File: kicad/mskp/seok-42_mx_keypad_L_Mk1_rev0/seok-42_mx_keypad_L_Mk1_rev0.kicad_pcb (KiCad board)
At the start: 2 copper layers, 162 x 117 mm, 44 parts, among them J1 Conn_01x12_Socket, SW1 Switch, SW10 Switch, SW11 Switch, SW12 Switch, SW13 Switch, SW14 Switch, SW15 Switch, SW16 Switch, SW17 Switch, SW18 Switch, SW19 Switch, SW2 Switch, SW20 Switch, SW21 Switch, SW3 Switch, SW4 Switch, SW5 Switch, SW6 Switch, SW7 Switch, SW8 Switch, SW9 Switch

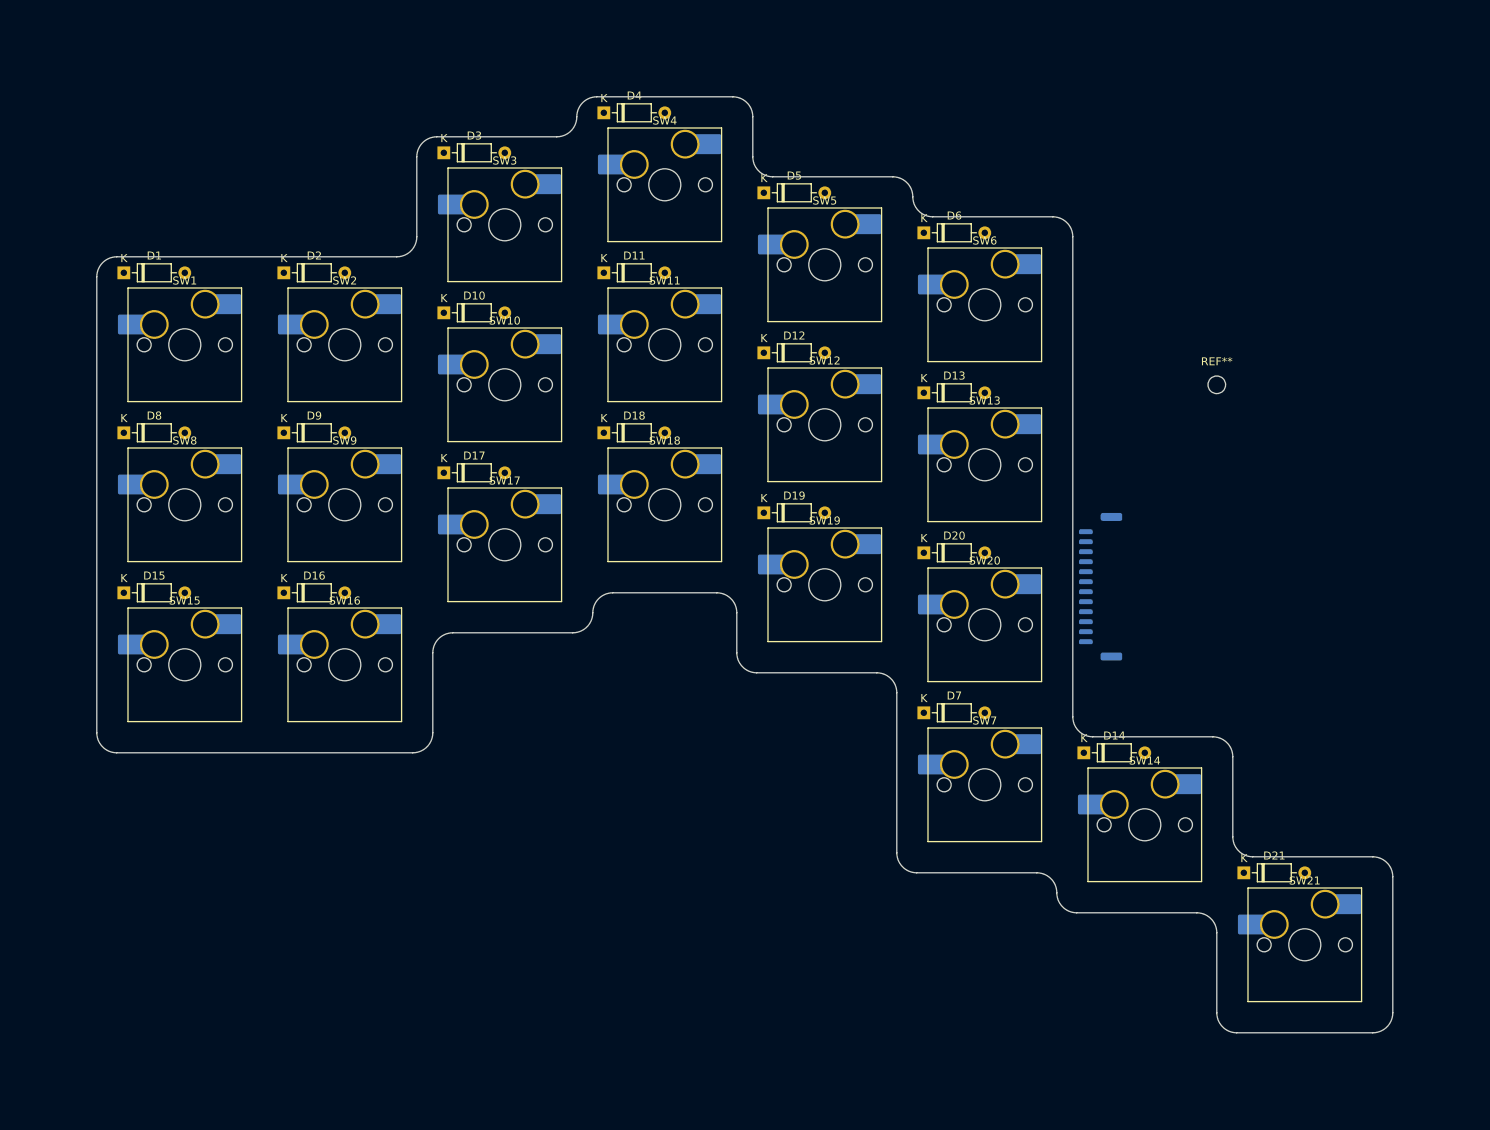
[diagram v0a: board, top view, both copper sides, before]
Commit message: Continues work with rough PCB outlines
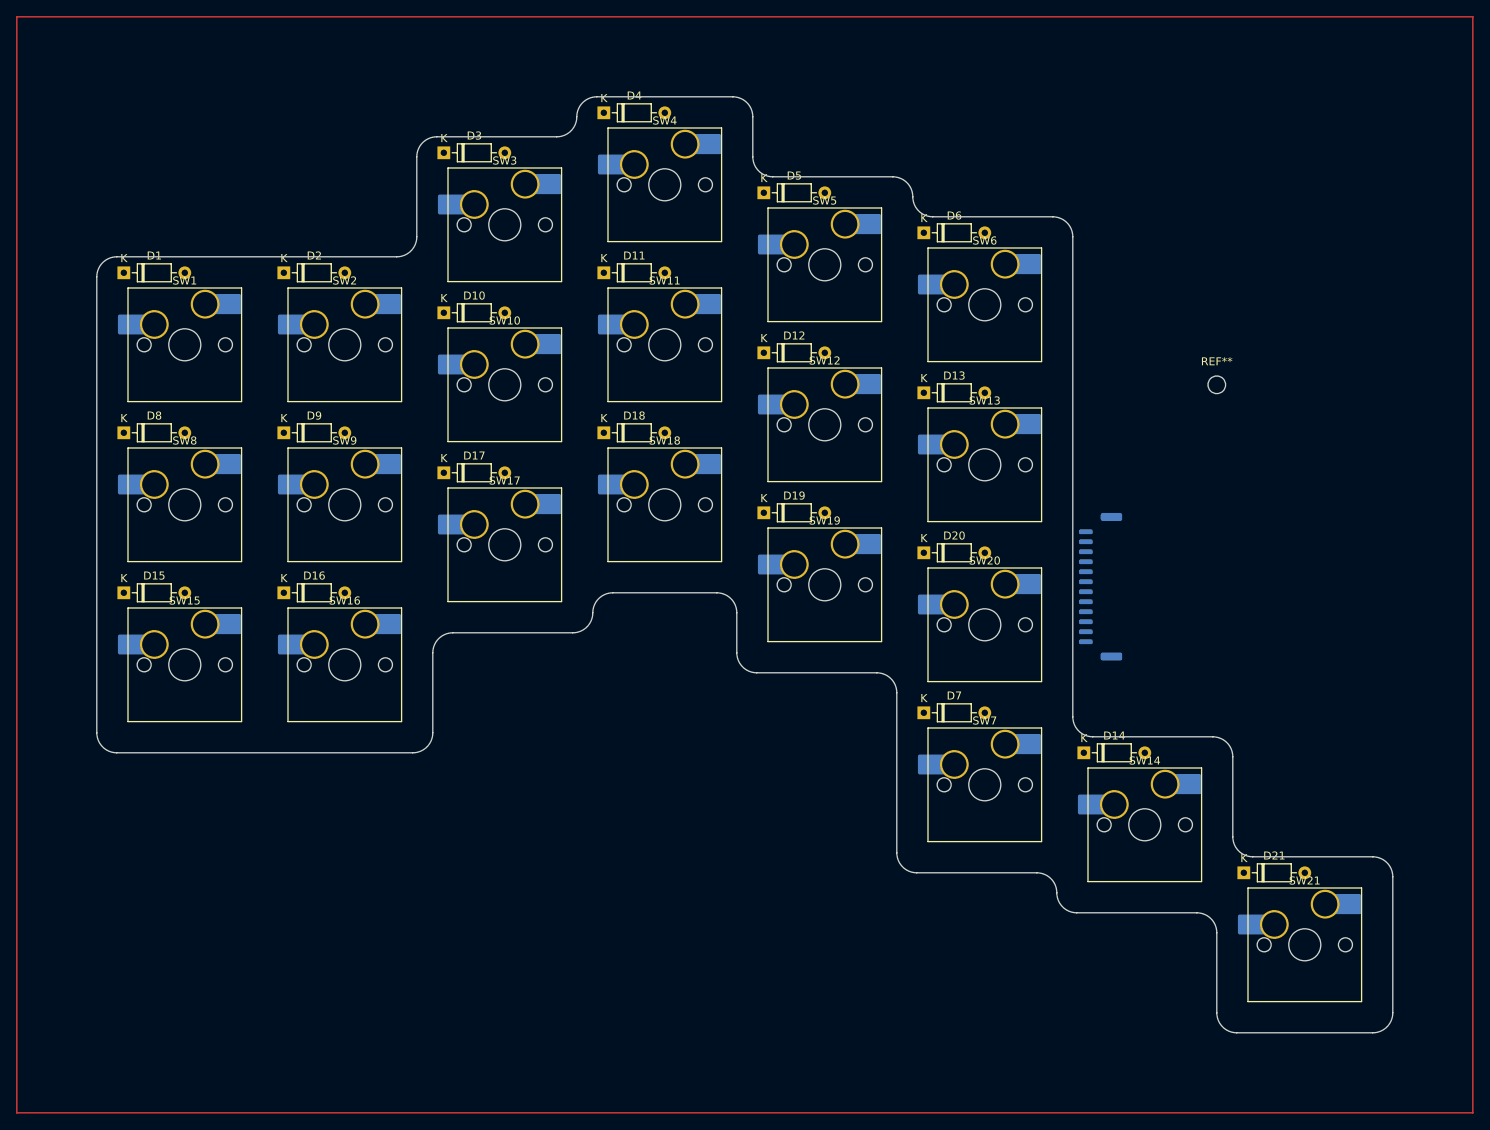
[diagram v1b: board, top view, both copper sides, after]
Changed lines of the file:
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@@
 		)
+	)
+	(gr_rect
+		(start 57 25)
+		(end 239 162)
+		(stroke
+			(width 0.2)
+			(type default)
+		)
+		(fill none)
+		(layer "F.Cu")
 	)
 	(gr_arc
@@
 		)
 		(layer "Edge.Cuts")
+	)
+	(dimension
+		(type aligned)
+		(layer "F.Cu")
+		(pts
+			(xy 218 152) (xy 218 162)
+		)
+		(height -6.75)
+		(gr_text "10.0000 mm"
+			(at 222.95 157 90)
+			(layer "F.Cu")
+			(effects
+				(font
+					(size 1.5 1.5)
+					(thickness 0.3)
+				)
+			)
+		)
+		(format
+			(prefix "")
+			(suffix "")
+			(units 3)
+			(units_format 1)
+			(precision 4)
+		)
+		(style
+			(thickness 0.2)
+			(arrow_length 1.27)
+			(text_position_mode 0)
+			(extension_height 0.58642)
+			(extension_offset 0.5) keep_text_aligned)
 	)
 	(dimension
@@
 			(layer "F.Cu")
 			(effects
+				(font
+					(size 1.5 1.5)
+					(thickness 0.3)
+				)
+			)
+		)
+		(format
+			(prefix "")
+			(suffix "")
+			(units 3)
+			(units_format 1)
+			(precision 4)
+		)
+		(style
+			(thickness 0.2)
+			(arrow_length 1.27)
+			(text_position_mode 0)
+			(extension_height 0.58642)
+			(extension_offset 0.5) keep_text_aligned)
+	)
+	(dimension
+		(type aligned)
+		(layer "F.Cu")
+		(pts
+			(xy 138 35) (xy 138 25)
+		)
+		(height 5.5)
+		(gr_text "10.0000 mm"
+			(at 141.7 30 90)
+			(layer "F.Cu")
+			(effects
